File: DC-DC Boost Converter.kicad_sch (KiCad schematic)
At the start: 13 parts, among them J1 Conn_01x01_Pin, J2 Conn_01x01_Pin, J3 Conn_01x01_Pin, J4 Conn_01x01_Pin

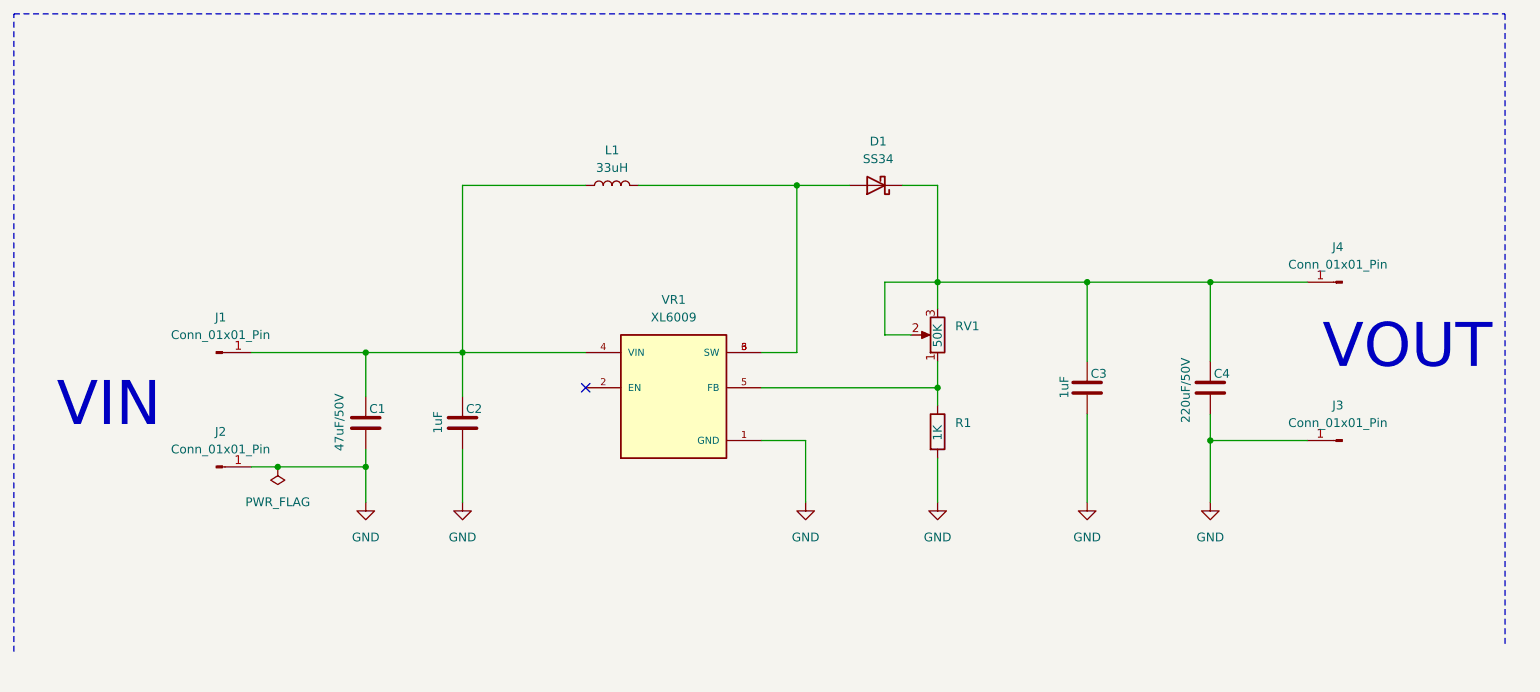
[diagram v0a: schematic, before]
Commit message: Final Schematic
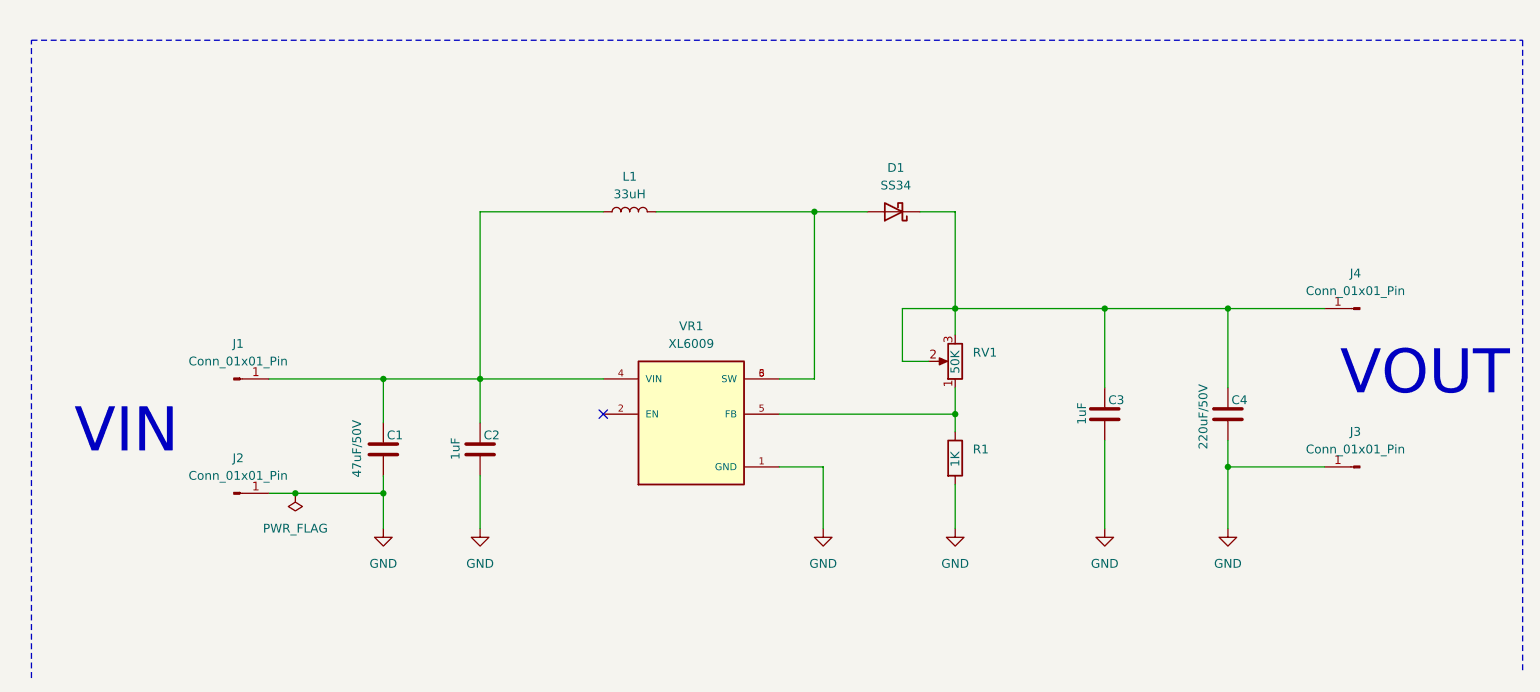
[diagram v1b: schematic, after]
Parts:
- C1, C4: footprint (none) -> Capacitor_THT:C_Radial_D6.3mm_H11.0mm_P2.50mm
- C2, C3: footprint (none) -> Capacitor_SMD:C_0805_2012Metric
- J1, J2, J3, J4: footprint (none) -> Connector_PinHeader_2.54mm:PinHeader_1x01_P2.54mm_Vertical
- L1: footprint (none) -> Inductor_SMD:L_12x12mm_H8mm
- R1: footprint (none) -> Resistor_SMD:R_1206_3216Metric
- RV1: footprint (none) -> Potentiometer_THT:Potentiometer_Bourns_3296W_Vertical
- VR1: footprint XL6009:DPAK170P1435X465-6N -> Footprints:DPAK170P1435X465-6N
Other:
- moved on the sheet: C1, C2, C3, C4, D1, J1, J2, J3, J4, L1, R1, RV1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
